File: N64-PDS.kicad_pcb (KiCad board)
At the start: 2 copper layers, 35.5 x 59.8 mm, 64 parts, among them J1 USB-C-6P-PWR, J2 I2C_OUT, J3 PWR_OUT, U1 STUSB4500QTR, U2 PTPS55289RYQR, U3 STL6P3LLH6, U4 PTPS55289RYQR

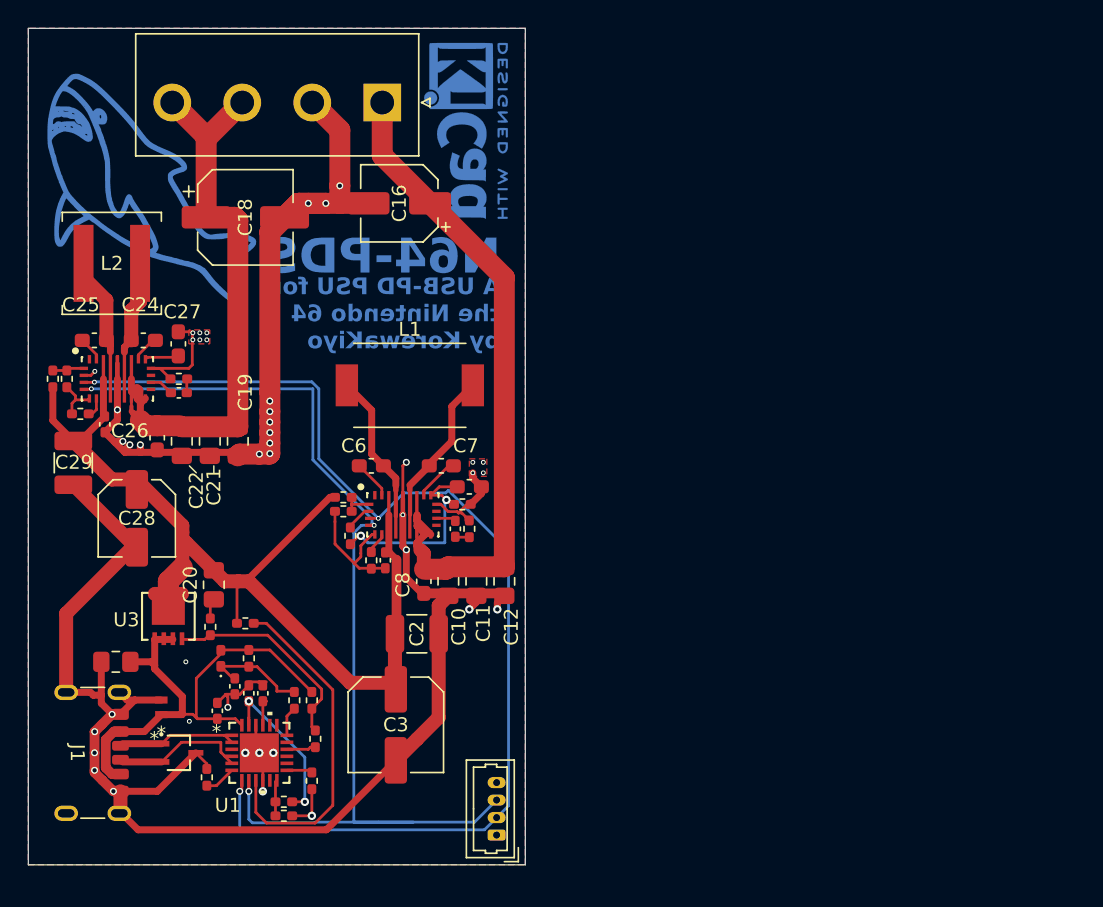
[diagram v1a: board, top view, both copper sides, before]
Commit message: Oops all redesigns
I did it again, this time smaller, better laid out, and all around maybe gooderer
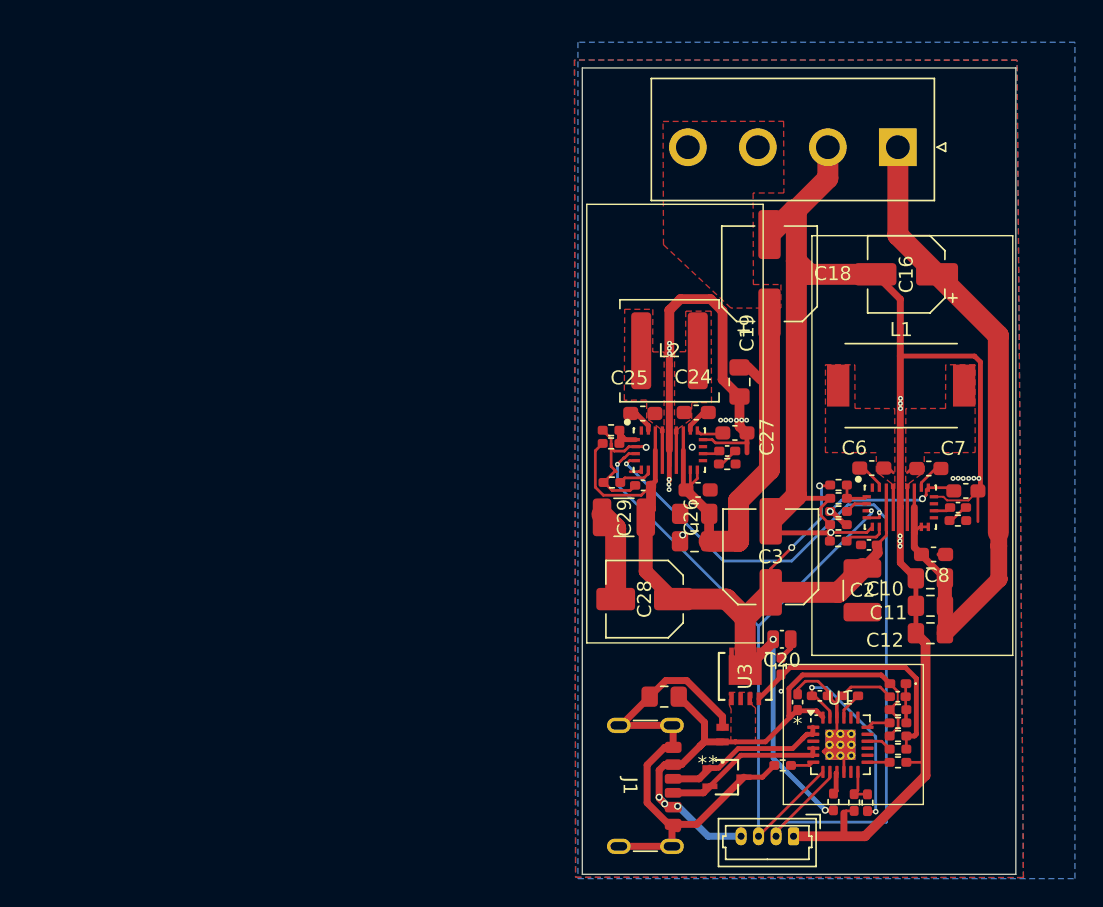
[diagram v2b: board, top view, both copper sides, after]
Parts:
- removed C9: 100n, Capacitor_SMD:C_0402_1005Metric_Pad0.74x0.62mm_HandSolder
- added C32: 4.7n, Capacitor_SMD:C_0402_1005Metric_Pad0.74x0.62mm_HandSolder, F.Cu at (200.4, 100.0)
- added kibuzzard-682FAEAC: G***, kibuzzard-682FAEAC, F.Cu at (201.0, 116.6)
- added kibuzzard-682FAEBC: G***, kibuzzard-682FAEBC, F.Cu at (192.6, 124.4)
- added kibuzzard-682FAEC4: G***, kibuzzard-682FAEC4, F.Cu at (175.5, 112.0)
- added kibuzzard-682FAECA: G***, kibuzzard-682FAECA, F.Cu at (201.6, 112.7)
- added kibuzzard-682FAF07: G***, kibuzzard-682FAF07, F.Cu at (201.1, 74.4)
- added kibuzzard-682FAF0F: G***, kibuzzard-682FAF0F, F.Cu at (176.4, 74.6)
- added kibuzzard-682FAF25: G***, kibuzzard-682FAF25, F.Cu at (191.1, 70.9)
- C20: footprint Capacitor_SMD:C_0805_2012Metric_Pad1.18x1.45mm_HandSolder -> Capacitor_SMD:C_0504_1310Metric_Pad0.83x1.28mm_HandSolder
- R20: value 274 -> 274k
- R9: value 301 -> 56.2k
- U1: footprint STUSB4500:QFN24EP_4X4_STM-M -> Package_DFN_QFN:QFN-24-1EP_4x4mm_P0.5mm_EP2.15x2.15mm_ThermalVias
- moved REF** 57.2 mm to (200.4, 118.4), turned to 90 degrees
- moved D1 48.4 mm to (196.1, 112.6), turned to 180 degrees
- moved C13 47.4 mm to (196.1, 113.5), turned to 0 degrees
- moved R12 46.5 mm to (196.1, 114.4), turned to 0 degrees
- moved R16 43.9 mm to (191.5, 121.0), turned to -90 degrees
- moved G*** 43.9 mm to (185.3, 87.5)
- moved R13 43.2 mm to (196.1, 115.4), turned to 180 degrees
- moved C15 42.0 mm to (192.7, 113.4), turned to 180 degrees
- moved R14 41.9 mm to (196.1, 116.3), turned to 0 degrees
- moved R10 41.9 mm to (196.1, 118.2), turned to 0 degrees
- moved R5 41.7 mm to (193.9, 121.1), turned to -90 degrees
- moved R11 41.6 mm to (196.1, 117.2), turned to 0 degrees
- moved U1 41.5 mm to (192.0, 116.9)
- moved C17 41.5 mm to (188.9, 113.9)
- moved U3 41.4 mm to (185.2, 112.0)
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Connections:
- net DISCH renamed /DISCH
- J2 pad 2: I2C_SCL -> /I2C_SDA
- J2 pad 3: I2C_SDA -> /I2C_SCL
- J2 pad 4: I2C_3V3 -> /VBUS
- R3 pad 1: GND -> Net-(U1-RESET)
- R3 pad 2: Net-(U1-RESET) -> GND
- U1 pad 7: I2C_SCL -> /I2C_SCL
- U1 pad 8: I2C_SDA -> /I2C_SDA
- U2 pad 3: I2C_SCL -> /I2C_SCL
- U2 pad 4: I2C_SDA -> /I2C_SDA
- U4 pad 3: I2C_SCL -> /I2C_SCL
- U4 pad 4: I2C_SDA -> /I2C_SDA
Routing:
- net I2C_SCL: track 82.3 -> 0.00 mm, vias 3 -> 0
- net I2C_SDA: track 76.6 -> 0.00 mm, vias 3 -> 0
- net /I2C_SDA: track 0.00 -> 61.4 mm, vias 0 -> 2
- net /I2C_SCL: track 0.00 -> 50.8 mm, vias 0 -> 2
- net GND: track 198.9 -> 227.6 mm, vias 43 -> 29
- net /DISCH: track 24.5 -> 1.54 mm
- net 3V3O: track 45.0 -> 30.6 mm
- net Net-(U2-SW2): track 11.1 -> 0.40 mm
- net Net-(U2-SW1): track 10.7 -> 0.43 mm
- net Net-(U4-SW2): track 8.71 -> 0.00 mm
- net Net-(U4-SW1): track 8.32 -> 0.00 mm
- net /VBUS: track 36.8 -> 43.1 mm, vias 0 -> 3
- net /VBUS_VS_DISCH: track 7.56 -> 3.72 mm
- net VSNK: track 74.8 -> 71.0 mm, vias 0 -> 4
- net Net-(U3-G): track 15.0 -> 18.2 mm
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- added copper zone on F.Cu, net /VBUS
- added copper zone on F.Cu, net 3V3O
- added copper zone on F.Cu, net Net-(U2-SW1)
- added copper zone on F.Cu, net Net-(U2-SW2)
- added copper zone on F.Cu, net Net-(U4-SW1)
- added copper zone on F.Cu, net Net-(U4-SW2)
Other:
- board size 35.5 x 59.8 mm -> 31 x 57.6 mm
